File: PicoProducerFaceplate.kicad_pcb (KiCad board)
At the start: 2 copper layers, 90 x 65 mm, 4 parts

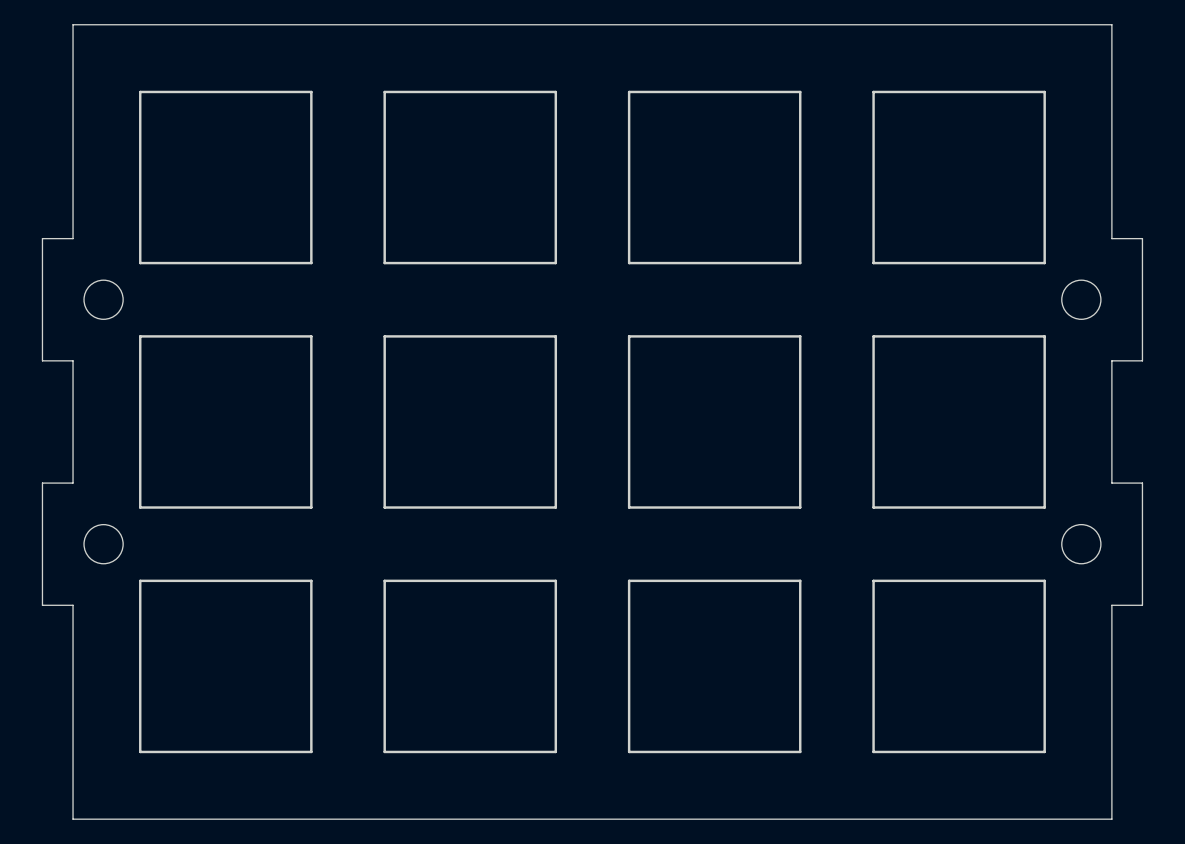
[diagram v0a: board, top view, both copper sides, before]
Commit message: 3dfiles
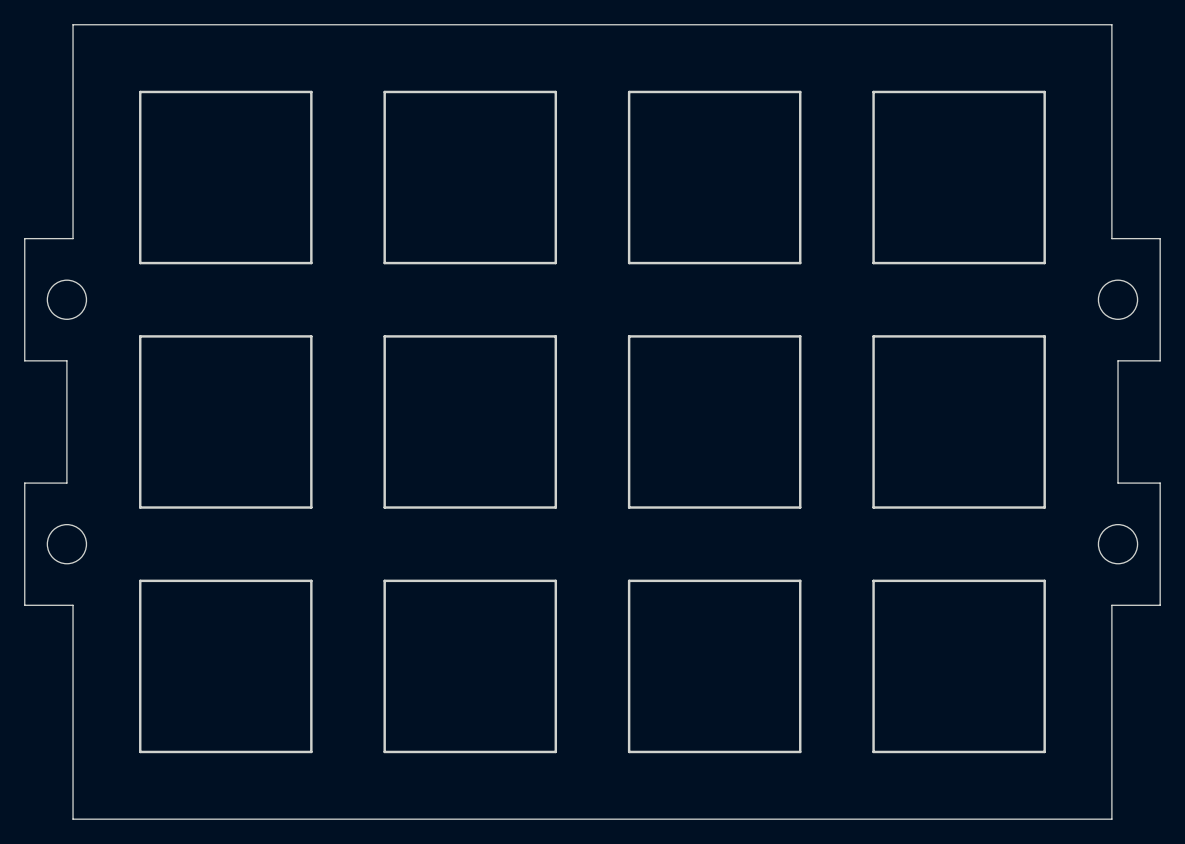
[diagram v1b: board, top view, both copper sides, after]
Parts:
- moved H1 3.00 mm to (17.0, 40.0)
- moved H2 3.00 mm to (103.0, 40.0)
- moved H3 3.00 mm to (17.0, 60.0)
- moved H4 3.00 mm to (103.0, 60.0)
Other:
- board size 90 x 65 mm -> 92.9 x 65 mm
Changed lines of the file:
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@@
 	(footprint "MountingHole:MountingHole_3.2mm_M3"
 		(layer "F.Cu")
-		(at 20 60)
+		(at 17 60)
 		(descr "Mounting Hole 3.2mm, no annular, M3")
 		(tags "mounting hole 3.2mm no annular m3")
@@
 	(footprint "MountingHole:MountingHole_3.2mm_M3"
 		(layer "F.Cu")
-		(at 100 60)
+		(at 103 60)
 		(descr "Mounting Hole 3.2mm, no annular, M3")
 		(tags "mounting hole 3.2mm no annular m3")
@@
 	(footprint "MountingHole:MountingHole_3.2mm_M3"
 		(layer "F.Cu")
-		(at 100 40)
+		(at 103 40)
 		(descr "Mounting Hole 3.2mm, no annular, M3")
 		(tags "mounting hole 3.2mm no annular m3")
@@
 	(footprint "MountingHole:MountingHole_3.2mm_M3"
 		(layer "F.Cu")
-		(at 20 40)
+		(at 17 40)
 		(descr "Mounting Hole 3.2mm, no annular, M3")
 		(tags "mounting hole 3.2mm no annular m3")
@@
 	)
 	(gr_line
-		(start 15 45)
-		(end 17.5 45)
+		(start 13.55 45)
+		(end 17 45)
 		(stroke
 			(width 0.05)
@@
 	)
 	(gr_line
-		(start 15 55)
-		(end 15 65)
+		(start 13.55 55)
+		(end 13.55 65)
 		(stroke
 			(width 0.05)
@@
 	(gr_line
 		(start 17.5 35)
-		(end 15 35)
+		(end 13.55 35)
 		(stroke
 			(width 0.05)
@@
 	)
 	(gr_line
-		(start 105 55)
-		(end 105 65)
+		(start 106.45 55)
+		(end 106.45 65)
 		(stroke
 			(width 0.05)
@@
 	)
 	(gr_line
-		(start 105 35)
-		(end 105 45)
-		(stroke
-			(width 0.05)
-			(type default)
-		)
-		(layer "Edge.Cuts")
-	)
-	(gr_line
-		(start 102.5 55)
-		(end 105 55)
+		(start 106.45 35)
+		(end 106.45 45)
+		(stroke
+			(width 0.05)
+			(type default)
+		)
+		(layer "Edge.Cuts")
+	)
+	(gr_line
+		(start 103 55)
+		(end 106.45 55)
 		(stroke
 			(width 0.05)
@@
 	)
 	(gr_line
-		(start 102.5 45)
-		(end 102.5 55)
+		(start 103 45)
+		(end 103 55)
 		(stroke
 			(width 0.05)
@@
 	(gr_line
 		(start 102.5 35)
-		(end 105 35)
+		(end 106.45 35)
 		(stroke
 			(width 0.05)
@@
 	)
 	(gr_line
-		(start 105 45)
-		(end 102.5 45)
+		(start 106.45 45)
+		(end 103 45)
 		(stroke
 			(width 0.05)
@@
 	)
 	(gr_line
-		(start 105 65)
+		(start 106.45 65)
 		(end 102.5 65)
 		(stroke
@@
 	)
 	(gr_line
-		(start 17.5 45)
-		(end 17.5 55)
-		(stroke
-			(width 0.05)
-			(type default)
-		)
-		(layer "Edge.Cuts")
-	)
-	(gr_line
-		(start 15 65)
+		(start 17 45)
+		(end 17 55)
+		(stroke
+			(width 0.05)
+			(type default)
+		)
+		(layer "Edge.Cuts")
+	)
+	(gr_line
+		(start 13.55 65)
 		(end 17.5 65)
 		(stroke
@@
 	)
 	(gr_line
-		(start 15 35)
-		(end 15 45)
+		(start 13.55 35)
+		(end 13.55 45)
 		(stroke
 			(width 0.05)
@@
 	)
 	(gr_line
-		(start 17.5 55)
-		(end 15 55)
-		(stroke
-			(width 0.05)
+		(start 17 55)
+		(end 13.55 55)
+		(stroke
+			(width 0.05)
